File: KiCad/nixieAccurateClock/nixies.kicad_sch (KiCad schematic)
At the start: 7 parts, among them J9 Conn_02x05_Odd_Even

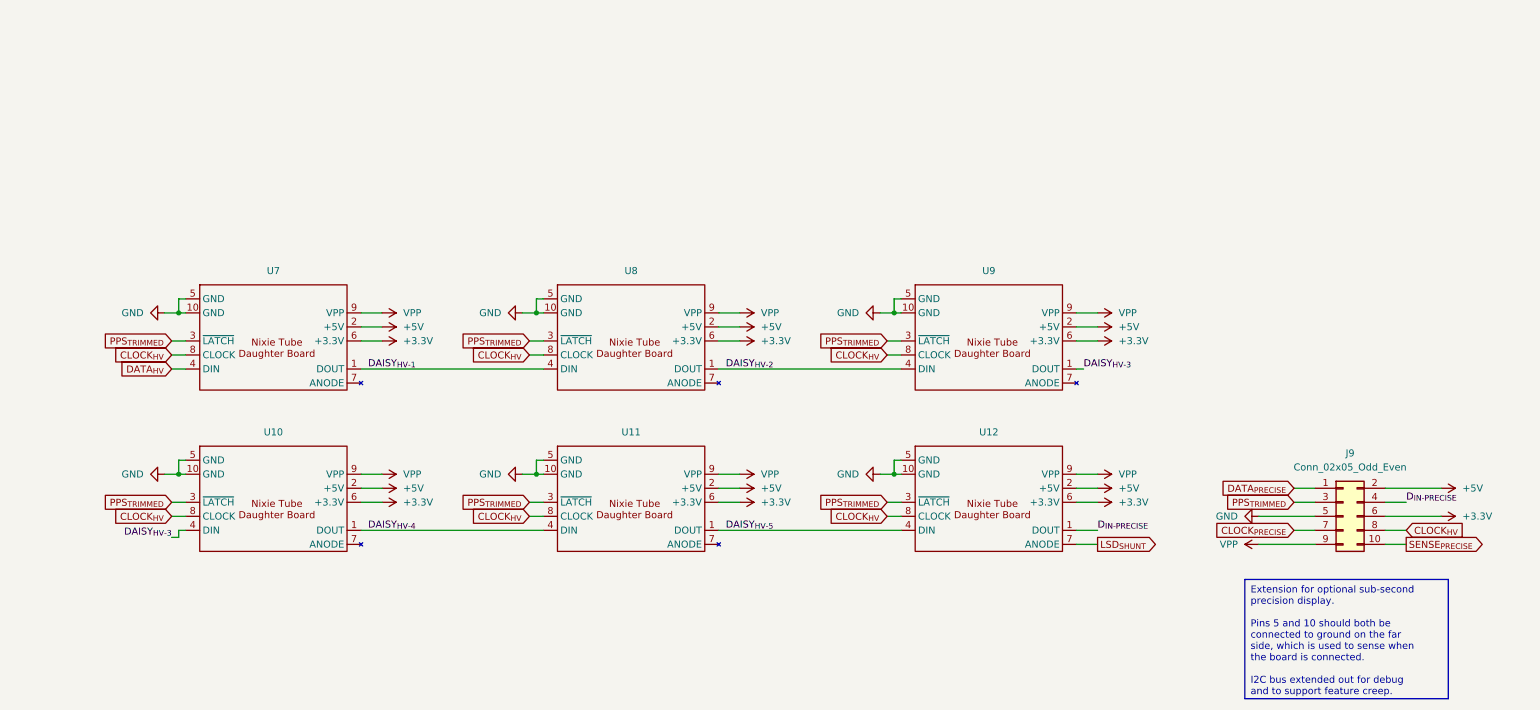
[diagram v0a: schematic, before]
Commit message: Add retailer links
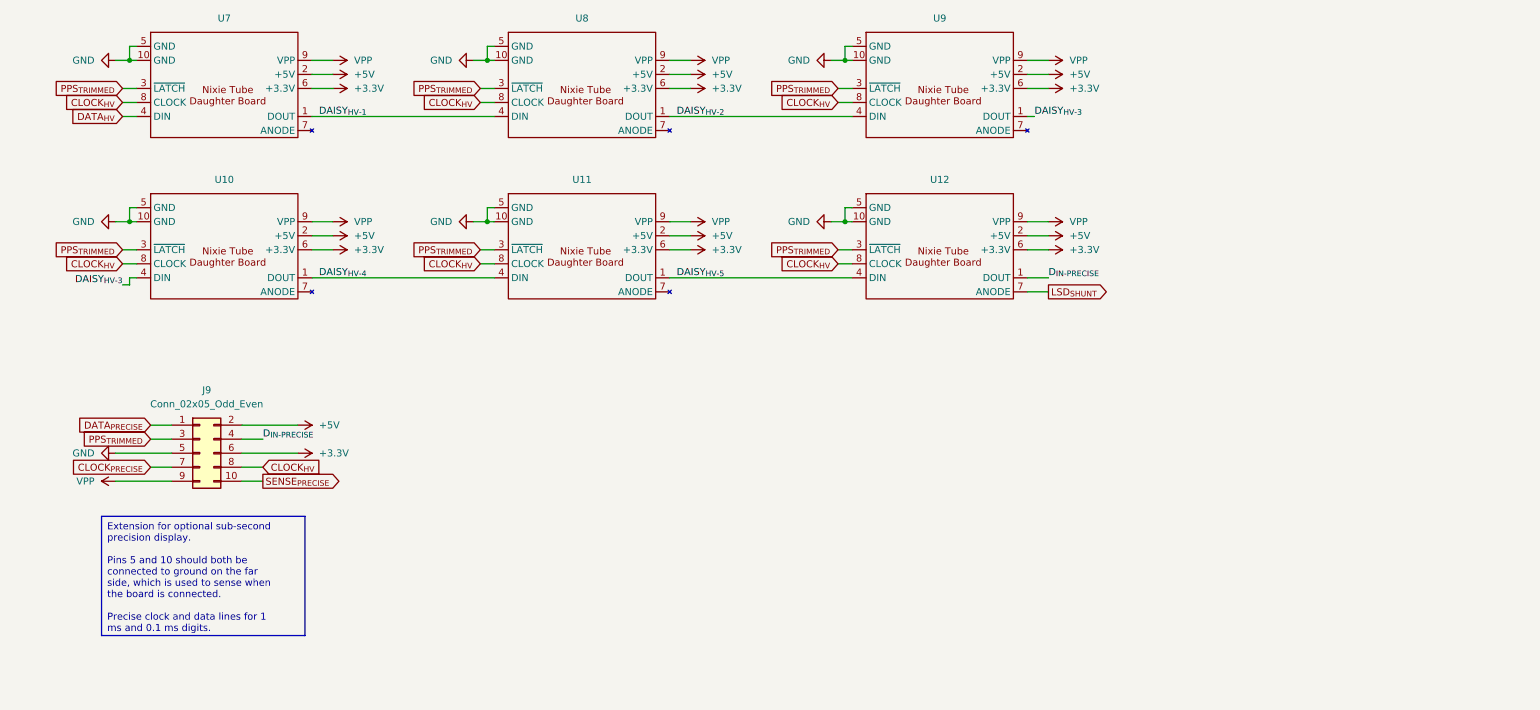
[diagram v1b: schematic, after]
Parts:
- J9: Digikey link (none) -> https://www.digikey.com/en/products/detail/sullins-connecto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; Mouser link (none) -> N/A
- U10, U11, U12, U7, U8, U9: Digikey link (none) -> N/A; Mouser link (none) -> N/A
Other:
- moved on the sheet: J9, U10, U11, U12, U7, U8, U9
